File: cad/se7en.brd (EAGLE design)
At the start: 64 x 34 mm, 67 parts, among them CN1 MICROSD-EJECT, CN3 DO NOT PLACE, CN4 DO NOT PLACE, CN5 DO NOT PLACE, CN6 DO NOT PLACE, CN7 DO NOT PLACE, Q1 FDC6329S, SW1 SWITCHKMR211, SW2 SWITCHKMR211, U1 ATSAME70, U2 MCP73831, X1 12MHz, X2 32k768

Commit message: tweak
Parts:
- U1: value ATSAME70 -> ATSAMS70
- renumbered LOGO1 to LOGO$1
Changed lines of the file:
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@@
 <grid distance="0.1" unitdist="mm" unit="mm" style="lines" multiple="5" display="yes" altdistance="0.025" altunitdist="inch" altunit="inch"/>
 <layers>
-<layer number="1" name="Top" color="4" fill="1" visible="yes" active="yes"/>
+<layer number="1" name="Top" color="4" fill="1" visible="no" active="yes"/>
 <layer number="2" name="Route2" color="6" fill="1" visible="no" active="yes"/>
 <layer number="3" name="Route3" color="4" fill="3" visible="no" active="no"/>
 <layer number="14" name="Route14" color="1" fill="6" visible="no" active="no"/>
 <layer number="15" name="Route15" color="13" fill="1" visible="no" active="yes"/>
-<layer number="16" name="Bottom" color="1" fill="1" visible="yes" active="yes"/>
+<layer number="16" name="Bottom" color="1" fill="1" visible="no" active="yes"/>
 <layer number="17" name="Pads" color="2" fill="1" visible="yes" active="yes"/>
 <layer number="18" name="Vias" color="2" fill="1" visible="yes" active="yes"/>
@@
 <layer number="23" name="tOrigins" color="15" fill="1" visible="yes" active="yes"/>
 <layer number="24" name="bOrigins" color="15" fill="1" visible="yes" active="yes"/>
-<layer number="25" name="tNames" color="7" fill="1" visible="no" active="yes"/>
+<layer number="25" name="tNames" color="7" fill="1" visible="yes" active="yes"/>
 <layer number="26" name="bNames" color="7" fill="1" visible="yes" active="yes"/>
 <layer number="27" name="tValues" color="7" fill="1" visible="no" active="yes"/>
@@
 </autorouter>
 <elements>
-<element name="U1" library="jaw" package="TQFP-100-14X14MM" value="ATSAME70" x="89" y="53" smashed="yes">
+<element name="U1" library="jaw" package="TQFP-100-14X14MM" value="ATSAMS70" x="89" y="53" smashed="yes">
 <attribute name="NAME" x="79.5" y="60" size="1" layer="25" ratio="10"/>
 <attribute name="VALUE" x="85" y="49" size="1" layer="27" ratio="10"/>
@@
 <element name="U$1" library="jaw" package="ROBOTMAN-LOGO2" value="ROBOTMAN-LOGO2" x="91.2" y="58.4" rot="MR0"/>
 <element name="U$3" library="jaw" package="ROBOTMAN-LOGO2" value="ROBOTMAN-LOGO2" x="70.1" y="48"/>
-<element name="LOGO1" library="SparkFun-Aesthetics" package="OSHW-LOGO-M" value="OSHW-LOGOM" x="97.9" y="55.7" rot="MR0"/>
+<element name="LOGO$1" library="SparkFun-Aesthetics" package="OSHW-LOGO-M" value="OSHW-LOGOM" x="97.9" y="55.7" rot="MR0"/>
 <element name="U2" library="jaw" package="SOT-23-5" value="MCP73831" x="59.5" y="60" smashed="yes" rot="R90">
 <attribute name="NAME" x="58.305" y="60.395" size="0.75" layer="25" ratio="10" rot="R180"/>

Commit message: fix typo
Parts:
- Q1: value FDC6329S -> FDC6392S
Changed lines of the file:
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@@
 <layer number="23" name="tOrigins" color="15" fill="1" visible="yes" active="yes"/>
 <layer number="24" name="bOrigins" color="15" fill="1" visible="yes" active="yes"/>
-<layer number="25" name="tNames" color="7" fill="1" visible="yes" active="yes"/>
+<layer number="25" name="tNames" color="7" fill="1" visible="no" active="yes"/>
 <layer number="26" name="bNames" color="7" fill="1" visible="yes" active="yes"/>
-<layer number="27" name="tValues" color="7" fill="1" visible="no" active="yes"/>
+<layer number="27" name="tValues" color="7" fill="1" visible="yes" active="yes"/>
 <layer number="28" name="bValues" color="7" fill="1" visible="yes" active="yes"/>
 <layer number="29" name="tStop" color="7" fill="3" visible="no" active="yes"/>
@@
 <attribute name="VALUE" x="100.122" y="33.714" size="1" layer="27" font="vector" ratio="10"/>
 </element>
-<element name="Q1" library="jaw" package="SOT-23-6" value="FDC6329S" x="63" y="60" smashed="yes" rot="R270">
+<element name="Q1" library="jaw" package="SOT-23-6" value="FDC6392S" x="63" y="60" smashed="yes" rot="R270">
 <attribute name="NAME" x="64.7" y="60.5" size="0.75" layer="25" ratio="10" rot="R270"/>
 <attribute name="VALUE" x="61.6" y="59.7" size="0.5" layer="27"/>

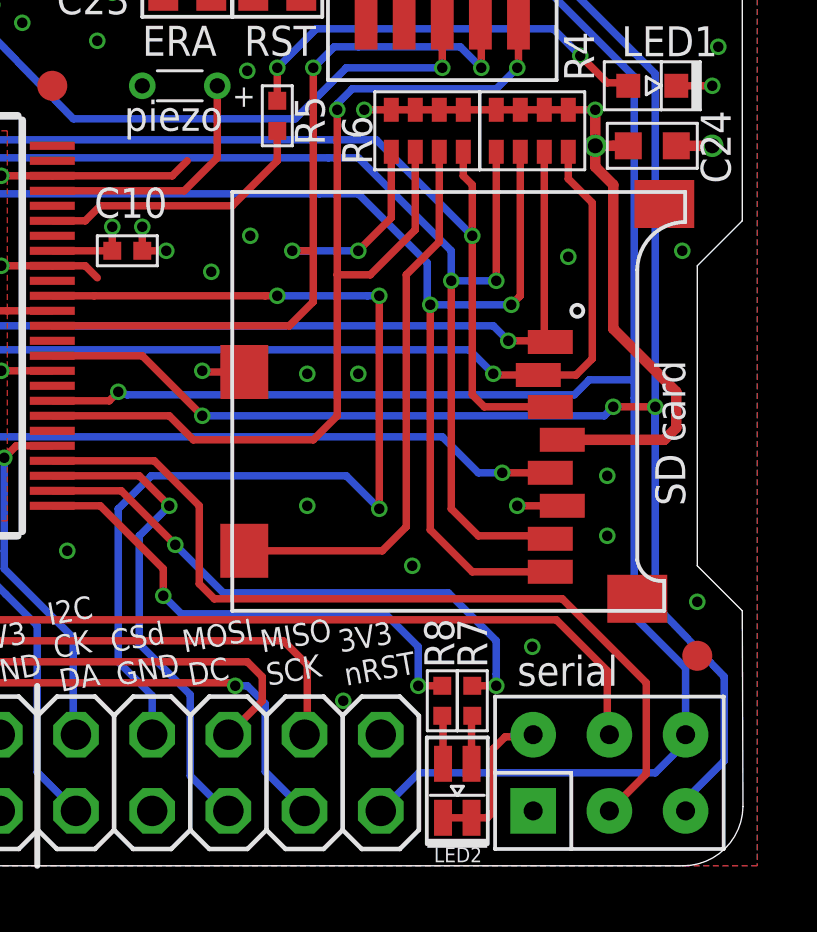
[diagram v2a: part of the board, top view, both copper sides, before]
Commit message: tweak orientation
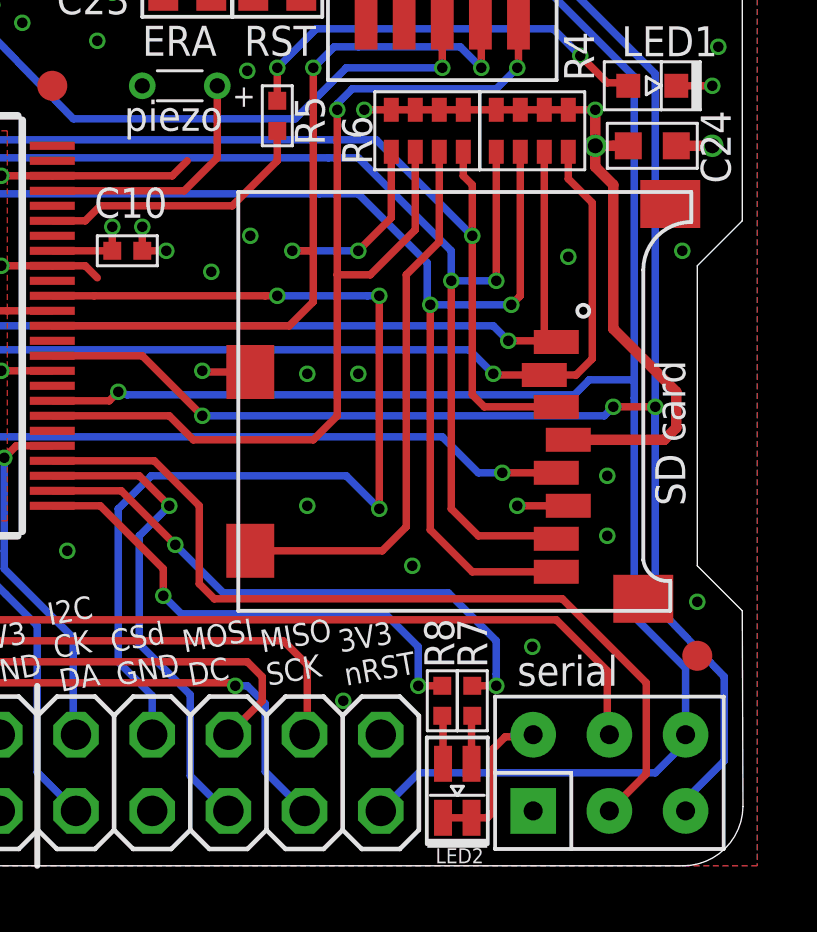
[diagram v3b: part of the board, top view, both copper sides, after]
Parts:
- moved CN1 0.50 mm to (110.0, 50.5), turned to 270 degrees
- turned LED2 to 90 degrees
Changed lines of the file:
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@@
 <grid distance="0.1" unitdist="mm" unit="mm" style="lines" multiple="5" display="yes" altdistance="0.025" altunitdist="inch" altunit="inch"/>
 <layers>
-<layer number="1" name="Top" color="4" fill="1" visible="no" active="yes"/>
+<layer number="1" name="Top" color="4" fill="1" visible="yes" active="yes"/>
 <layer number="2" name="Route2" color="6" fill="1" visible="no" active="yes"/>
 <layer number="3" name="Route3" color="4" fill="3" visible="no" active="no"/>
 <layer number="14" name="Route14" color="1" fill="6" visible="no" active="no"/>
 <layer number="15" name="Route15" color="13" fill="1" visible="no" active="yes"/>
-<layer number="16" name="Bottom" color="1" fill="1" visible="no" active="yes"/>
+<layer number="16" name="Bottom" color="1" fill="1" visible="yes" active="yes"/>
 <layer number="17" name="Pads" color="2" fill="1" visible="yes" active="yes"/>
 <layer number="18" name="Vias" color="2" fill="1" visible="yes" active="yes"/>
@@
 <layer number="23" name="tOrigins" color="15" fill="1" visible="yes" active="yes"/>
 <layer number="24" name="bOrigins" color="15" fill="1" visible="yes" active="yes"/>
-<layer number="25" name="tNames" color="7" fill="1" visible="no" active="yes"/>
+<layer number="25" name="tNames" color="7" fill="1" visible="yes" active="yes"/>
 <layer number="26" name="bNames" color="7" fill="1" visible="yes" active="yes"/>
-<layer number="27" name="tValues" color="7" fill="1" visible="yes" active="yes"/>
+<layer number="27" name="tValues" color="7" fill="1" visible="no" active="yes"/>
 <layer number="28" name="bValues" color="7" fill="1" visible="yes" active="yes"/>
 <layer number="29" name="tStop" color="7" fill="3" visible="no" active="yes"/>
@@
 <layer number="49" name="Reference" color="7" fill="1" visible="yes" active="yes"/>
 <layer number="50" name="dxf" color="7" fill="1" visible="no" active="no"/>
-<layer number="51" name="tDocu" color="7" fill="1" visible="no" active="yes"/>
+<layer number="51" name="tDocu" color="7" fill="1" visible="yes" active="yes"/>
 <layer number="52" name="bDocu" color="7" fill="1" visible="yes" active="yes"/>
 <layer number="53" name="tGND_GNDA" color="7" fill="1" visible="no" active="no"/>
@@
 <attribute name="VALUE" x="74" y="71" size="1.778" layer="27" rot="R180" display="off"/>
 </element>
-<element name="CN1" library="jaw" package="MICROSD/EJECTOR" value="MICROSD-EJECT" x="110.5" y="50.5" smashed="yes" rot="R90">
-<attribute name="NAME" x="107.1" y="47.2" size="1.27" layer="25" rot="R90" display="off"/>
+<element name="CN1" library="jaw" package="MICROSD/EJECTOR" value="MICROSD-EJECT" x="110" y="50.5" smashed="yes" rot="R270">
+<attribute name="NAME" x="113.4" y="53.8" size="1.27" layer="25" rot="R270" display="off"/>
 </element>
 <element name="C19" library="jaw" package="SMD0402" value=".1u" x="78" y="55.5" smashed="yes">
@@
 <attribute name="VALUE" x="110.4" y="41.9" size="1" layer="27" font="vector" ratio="10" rot="R90"/>
 </element>
-<element name="LED2" library="jaw" package="SMD0805-DUAL" value="LED-DUAL0805" x="110.5" y="37.5" smashed="yes" rot="R270">
-<attribute name="NAME" x="109.722" y="35.116" size="0.5" layer="25" font="vector" ratio="10"/>
-<attribute name="VALUE" x="100.122" y="33.714" size="1" layer="27" font="vector" ratio="10"/>
+<element name="LED2" library="jaw" package="SMD0805-DUAL" value="LED-DUAL0805" x="110.5" y="37.5" smashed="yes" rot="R90">
+<attribute name="NAME" x="111.378" y="35.584" size="0.5" layer="25" font="vector" ratio="10" rot="R180"/>
+<attribute name="VALUE" x="120.878" y="41.286" size="1" layer="27" font="vector" ratio="10" rot="R270" display="off"/>
 </element>
 <element name="Q1" library="jaw" package="SOT-23-6" value="FDC6392S" x="63" y="60" smashed="yes" rot="R270">
@@
 <contactref element="C24" pad="1"/>
 <via x="102" y="51.5" extent="1-16" drill="0.35"/>
-<wire x1="103.4" y1="51.46" x2="102.04" y2="51.46" width="0.25" layer="1"/>
+<wire x1="103.6" y1="51.46" x2="102.04" y2="51.46" width="0.25" layer="1"/>
 <wire x1="102.04" y1="51.46" x2="102" y2="51.5" width="0.25" layer="1"/>
 <via x="112.5" y="47" extent="1-16" drill="0.35"/>
-<wire x1="114" y1="47" x2="113.9" y2="47" width="0.25" layer="1"/>
+<wire x1="114.2" y1="47" x2="113.9" y2="47" width="0.25" layer="1"/>
 <wire x1="113.9" y1="47" x2="112.5" y2="47" width="0.25" layer="1"/>
 <contactref element="CN4" pad="3"/>
@@
 <via x="70" y="55" extent="1-16" drill="0.5"/>
 <via x="69.9" y="56.5" extent="1-16" drill="0.5"/>
-<wire x1="114" y1="49.2" x2="117.4" y2="49.2" width="0.35" layer="1"/>
+<wire x1="114.2" y1="49.2" x2="117.4" y2="49.2" width="0.35" layer="1"/>
 <wire x1="117.4" y1="49.2" x2="117.8" y2="49.6" width="0.35" layer="1"/>
 <wire x1="117.8" y1="49.6" x2="117.8" y2="50.8" width="0.35" layer="1"/>
@@
 <wire x1="110.3" y1="46.9" x2="111.2" y2="46" width="0.25" layer="1"/>
 <wire x1="111.2" y1="46" x2="113.5" y2="46" width="0.25" layer="1"/>
-<wire x1="113.5" y1="46" x2="113.6" y2="45.9" width="0.25" layer="1"/>
+<wire x1="113.5" y1="46" x2="113.8" y2="45.9" width="0.25" layer="1"/>
 <wire x1="111.8" y1="58.8" x2="111.8" y2="54.5" width="0.25" layer="1"/>
 <via x="111.8" y="54.5" extent="1-16" drill="0.35"/>
@@
 <wire x1="109.6" y1="53.7" x2="109.6" y2="46.2" width="0.25" layer="1"/>
 <wire x1="109.6" y1="46.2" x2="111" y2="44.8" width="0.25" layer="1"/>
-<wire x1="111" y1="44.8" x2="113.6" y2="44.8" width="0.25" layer="1"/>
+<wire x1="111" y1="44.8" x2="113.8" y2="44.8" width="0.25" layer="1"/>
 <wire x1="112.6" y1="58.8" x2="112.6" y2="54" width="0.25" layer="1"/>
 <wire x1="112.6" y1="54" x2="112.3" y2="53.7" width="0.25" layer="1"/>
@@
 <via x="112.2" y="52.5" extent="1-16" drill="0.35"/>
 <wire x1="112.2" y1="52.5" x2="113.56" y2="52.5" width="0.25" layer="1"/>
-<wire x1="113.56" y1="52.5" x2="113.6" y2="52.46" width="0.25" layer="1"/>
+<wire x1="113.56" y1="52.5" x2="113.8" y2="52.46" width="0.25" layer="1"/>
 <wire x1="91.5" y1="52.5" x2="92" y2="53" width="0.25" layer="16"/>
 <wire x1="92" y1="53" x2="111.7" y2="53" width="0.25" layer="16"/>
 <wire x1="111.7" y1="53" x2="112.2" y2="52.5" width="0.25" layer="16"/>
-<wire x1="113.4" y1="52.66" x2="113.6" y2="52.46" width="0.35" layer="1"/>
+<wire x1="113.4" y1="52.66" x2="113.8" y2="52.46" width="0.35" layer="1"/>
 <wire x1="113.4" y1="52.66" x2="113.4" y2="58.8" width="0.25" layer="1"/>
 </signal>
@@
 <via x="111.7" y="51.4" extent="1-16" drill="0.35"/>
 <wire x1="111.7" y1="51.4" x2="111.74" y2="51.36" width="0.25" layer="1"/>
-<wire x1="111.74" y1="51.36" x2="113.2" y2="51.36" width="0.25" layer="1"/>
-<wire x1="113.2" y1="51.36" x2="114.46" y2="51.36" width="0.25" layer="1"/>
+<wire x1="111.74" y1="51.36" x2="113.4" y2="51.36" width="0.25" layer="1"/>
+<wire x1="113.4" y1="51.36" x2="114.46" y2="51.36" width="0.25" layer="1"/>
 <wire x1="114.46" y1="51.36" x2="115" y2="51.9" width="0.25" layer="1"/>
 <wire x1="95" y1="45" x2="95" y2="46.5" width="0.25" layer="1"/>
@@
 <wire x1="111.9" y1="48" x2="112" y2="48.1" width="0.25" layer="16"/>
 <via x="112" y="48.1" extent="1-16" drill="0.35"/>
-<wire x1="112" y1="48.1" x2="113.6" y2="48.1" width="0.25" layer="1"/>
+<wire x1="112" y1="48.1" x2="113.8" y2="48.1" width="0.25" layer="1"/>
 <wire x1="90" y1="48" x2="91.3" y2="49.3" width="0.25" layer="16"/>
 <wire x1="91.3" y1="49.3" x2="110" y2="49.3" width="0.25" layer="16"/>
@@
 <wire x1="111" y1="56" x2="111" y2="50.7" width="0.25" layer="1"/>
 <wire x1="111" y1="50.7" x2="111.4" y2="50.3" width="0.25" layer="1"/>
-<wire x1="111.4" y1="50.3" x2="113.6" y2="50.3" width="0.25" layer="1"/>
+<wire x1="111.4" y1="50.3" x2="113.8" y2="50.3" width="0.25" layer="1"/>
 <contactref element="R6" pad="8"/>
 <wire x1="111" y1="56" x2="111" y2="57.7" width="0.25" layer="1"/>
@@
 <signal name="CARDIO">
 <contactref element="CN1" pad="CD1"/>
-<wire x1="108" y1="45.5" x2="103.4" y2="45.5" width="0.25" layer="1"/>
+<wire x1="108" y1="45.5" x2="103.6" y2="45.5" width="0.25" layer="1"/>
 <contactref element="R6" pad="7"/>
 <wire x1="109.9" y1="58.8" x2="109.9" y2="55.8" width="0.25" layer="1"/>
